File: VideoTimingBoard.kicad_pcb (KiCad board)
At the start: 2 copper layers, 66 x 38.1 mm, 43 parts, among them U1 MC44144, U2 LM1881, U3 SN74LVC3G04, U4 TLV3502

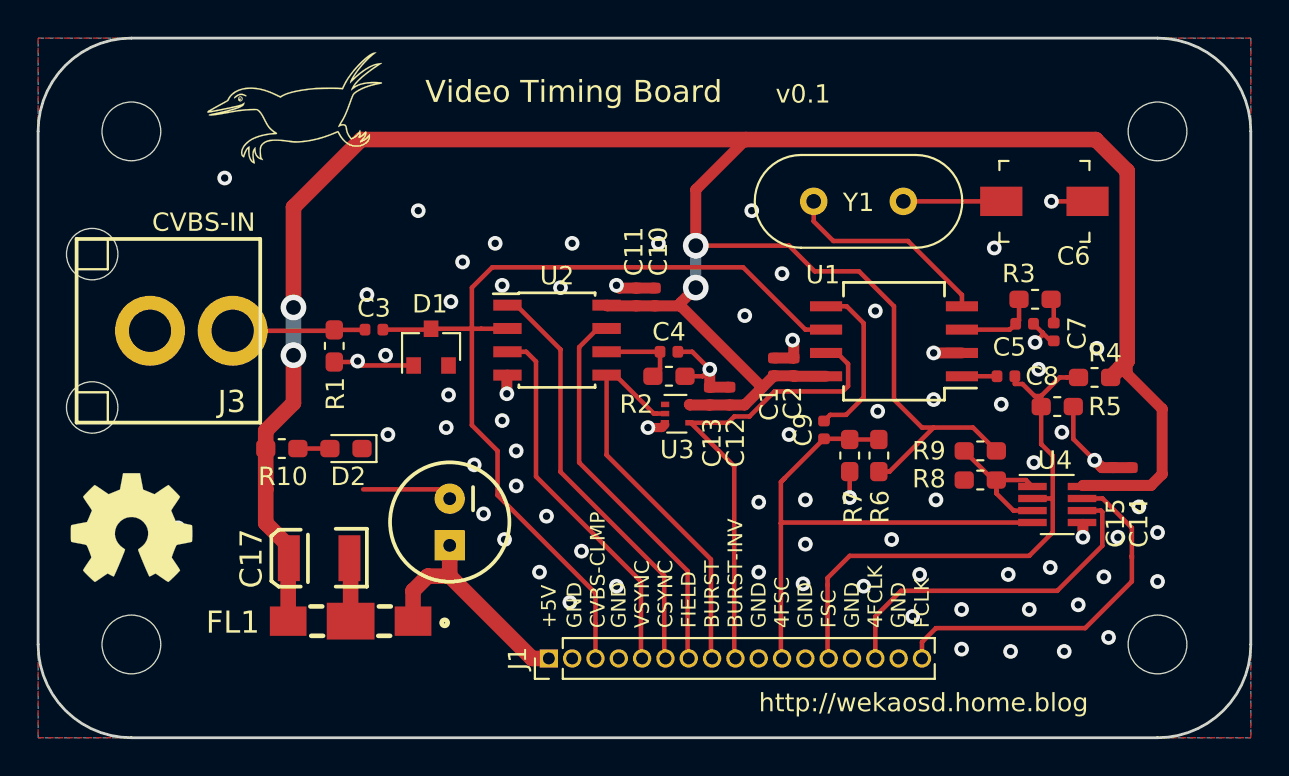
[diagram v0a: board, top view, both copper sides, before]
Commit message: Design complete.
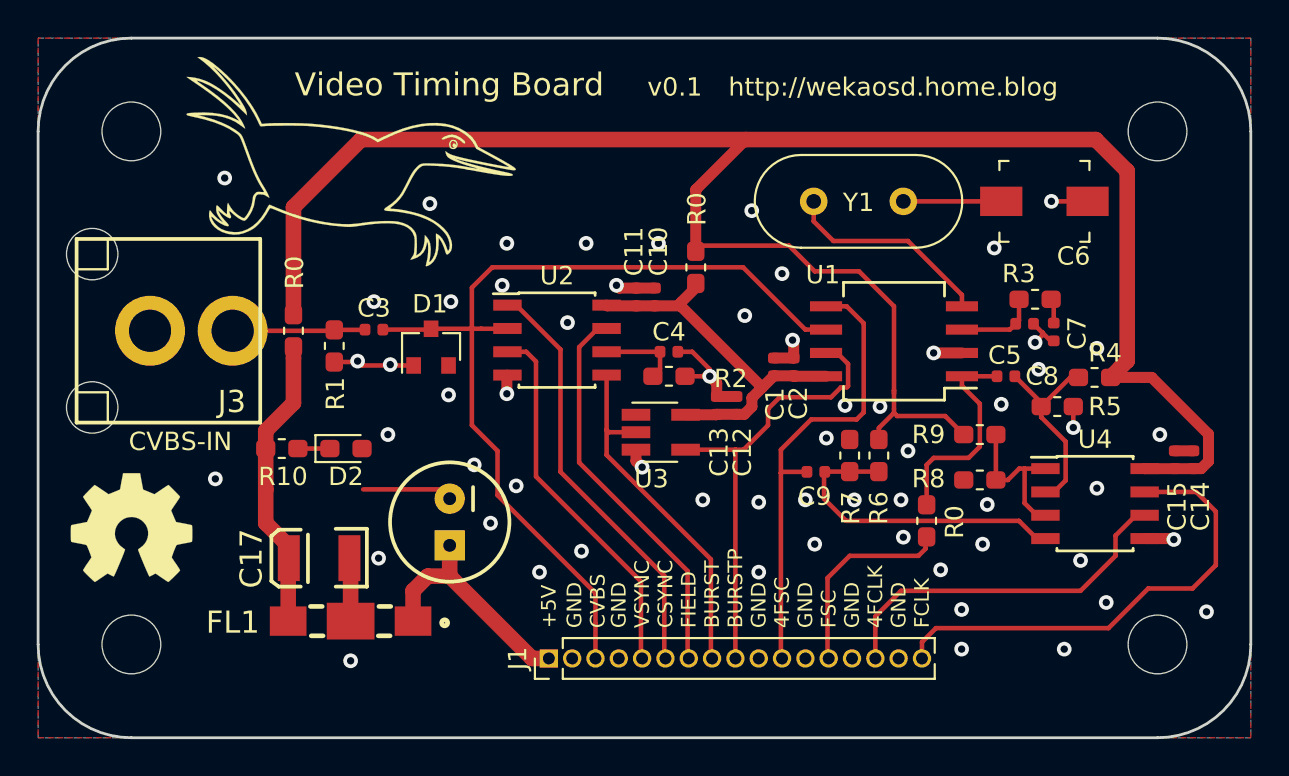
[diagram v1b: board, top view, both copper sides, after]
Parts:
- removed G***: LOGO, Footprints:weka_small
- added R0: 0R, Resistor_SMD:R_0603_1608Metric_Pad1.05x0.95mm_HandSolder, F.Cu at (148.8, 97.6)
- added R0: 0R, Resistor_SMD:R_0603_1608Metric_Pad1.05x0.95mm_HandSolder, F.Cu at (161.4, 111.4)
- added R0: 0R, Resistor_SMD:R_0603_1608Metric_Pad1.05x0.95mm_HandSolder, F.Cu at (126.9, 101.0)
- added ~: ~, Footprints:weka, F.Cu at (130.0, 91.8)
- C17: value ~ -> 33uF
- FL1: value ~ -> NFE61PT472C1H9L
- R10: value 10K -> 150R
- U3: value SN74LVC3G04 -> SN74LVC1GU04; footprint Package_SO:Texas_R-PDSO-N5 -> Package_TO_SOT_SMD:SOT-23-5_HandSoldering
- U4: value TLV3502 -> TLV3502AIDCNR; footprint Package_TO_SOT_SMD:SOT-23-8_Handsoldering -> Package_SO:SOIC-8_3.9x4.9mm_P1.27mm
- moved C14 3.48 mm to (175.9, 108.1)
- moved C15 3.48 mm to (174.9, 108.1)
- moved C9 2.33 mm to (155.4, 108.7), turned to 180 degrees
- moved U4 2.06 mm to (170.6, 110.4)
- moved U3 1.35 mm to (146.9, 106.6)
- moved R9 0.89 mm to (164.3, 106.7), turned to 180 degrees
- moved C12 0.63 mm to (151.1, 105.1)
- moved C13 0.63 mm to (150.0, 105.1)
- turned D2 to 0 degrees
- turned R6 to 270 degrees
- turned R7 to 90 degrees
- renumbered REF** to ~
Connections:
- C8 pad 1: /FSC -> /FSC-BIAS
- C8 pad 2: Net-(C8-Pad2) -> /FSC
- C9 pad 1: /4FSC -> /4FSC-BIAS
- C9 pad 2: Net-(C9-Pad2) -> /4FSC
- R4 pad 2: /FSC -> /FSC-BIAS
- R5 pad 1: /FSC -> /FSC-BIAS
- R6 pad 2: /4FSC -> /4FSC-BIAS
- R7 pad 1: /4FSC -> /4FSC-BIAS
- U1 pad 1: Net-(C8-Pad2) -> /FSC
- U1 pad 5: Net-(C9-Pad2) -> /4FSC
- U4 pad 2: /FSC -> /FSC-BIAS
- U4 pad 4: /4FSC -> /4FSC-BIAS
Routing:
- net /4FSC-BIAS: track 0.00 -> 17.4 mm
- net /FSC-BIAS: track 0.00 -> 10.9 mm
- net Net-(C9-Pad2): track 9.76 -> 0.00 mm
- net /FSC: track 31.1 -> 22.7 mm
- net VDD: track 151.4 -> 144.6 mm, vias 4 -> 0
- net /FCLK: track 20.1 -> 25.9 mm
- net /4FSC: track 29.8 -> 26.0 mm
- net GND: track 38.8 -> 35.2 mm, vias 75 -> 61
- net /BURST: track 22.3 -> 20.4 mm
- net Net-(C8-Pad2): track 1.91 -> 0.00 mm
- net Net-(R8-Pad2): track 7.44 -> 8.69 mm
- net /BURST-INV: track 26.0 -> 24.8 mm
- net /4FCLK: track 19.2 -> 19.9 mm
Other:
- board text added: "BURSTP"
- board text added: "CVBS"
- board text removed: "BURST-INV"
- board text removed: "CVBS-CLMP"
